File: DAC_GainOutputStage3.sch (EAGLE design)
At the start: 55 parts, among them J1 1935190, J3 SJ-63033A

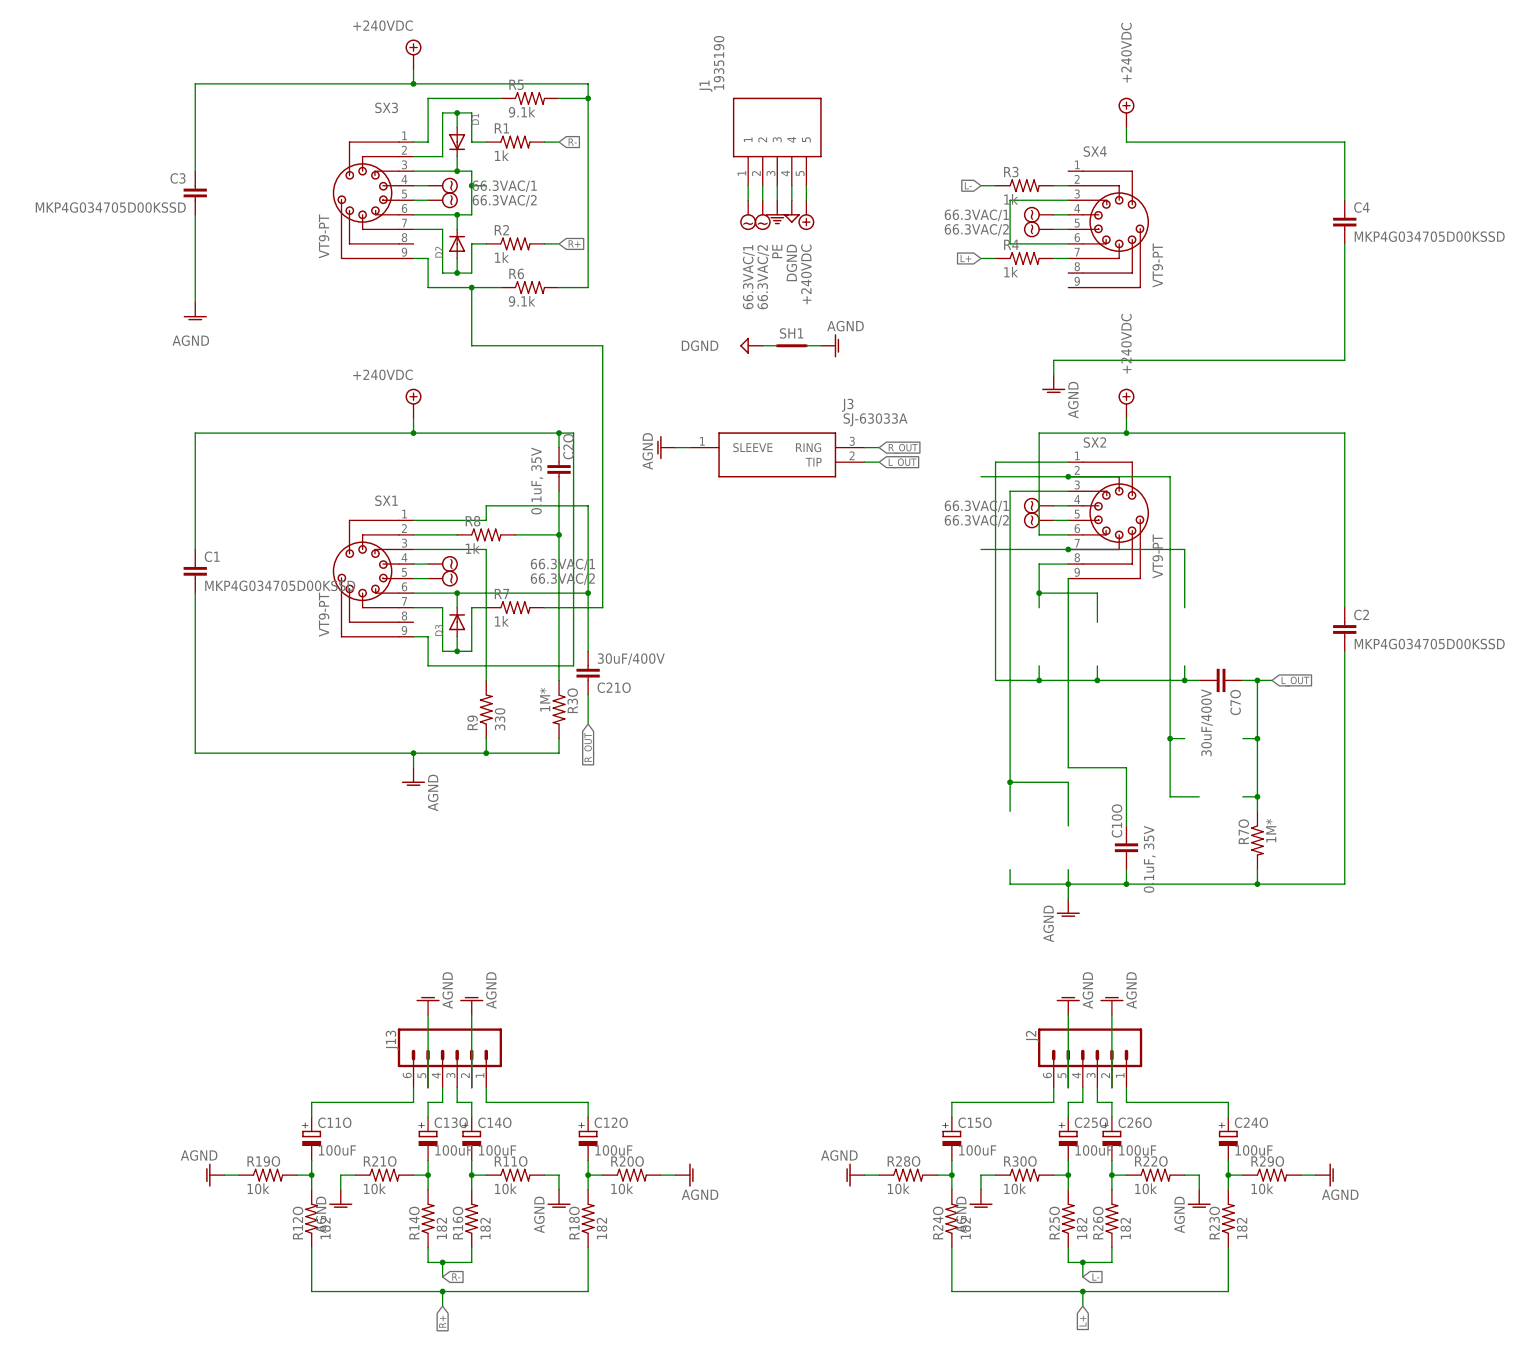
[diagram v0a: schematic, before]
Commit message: Finished schematic and working layout
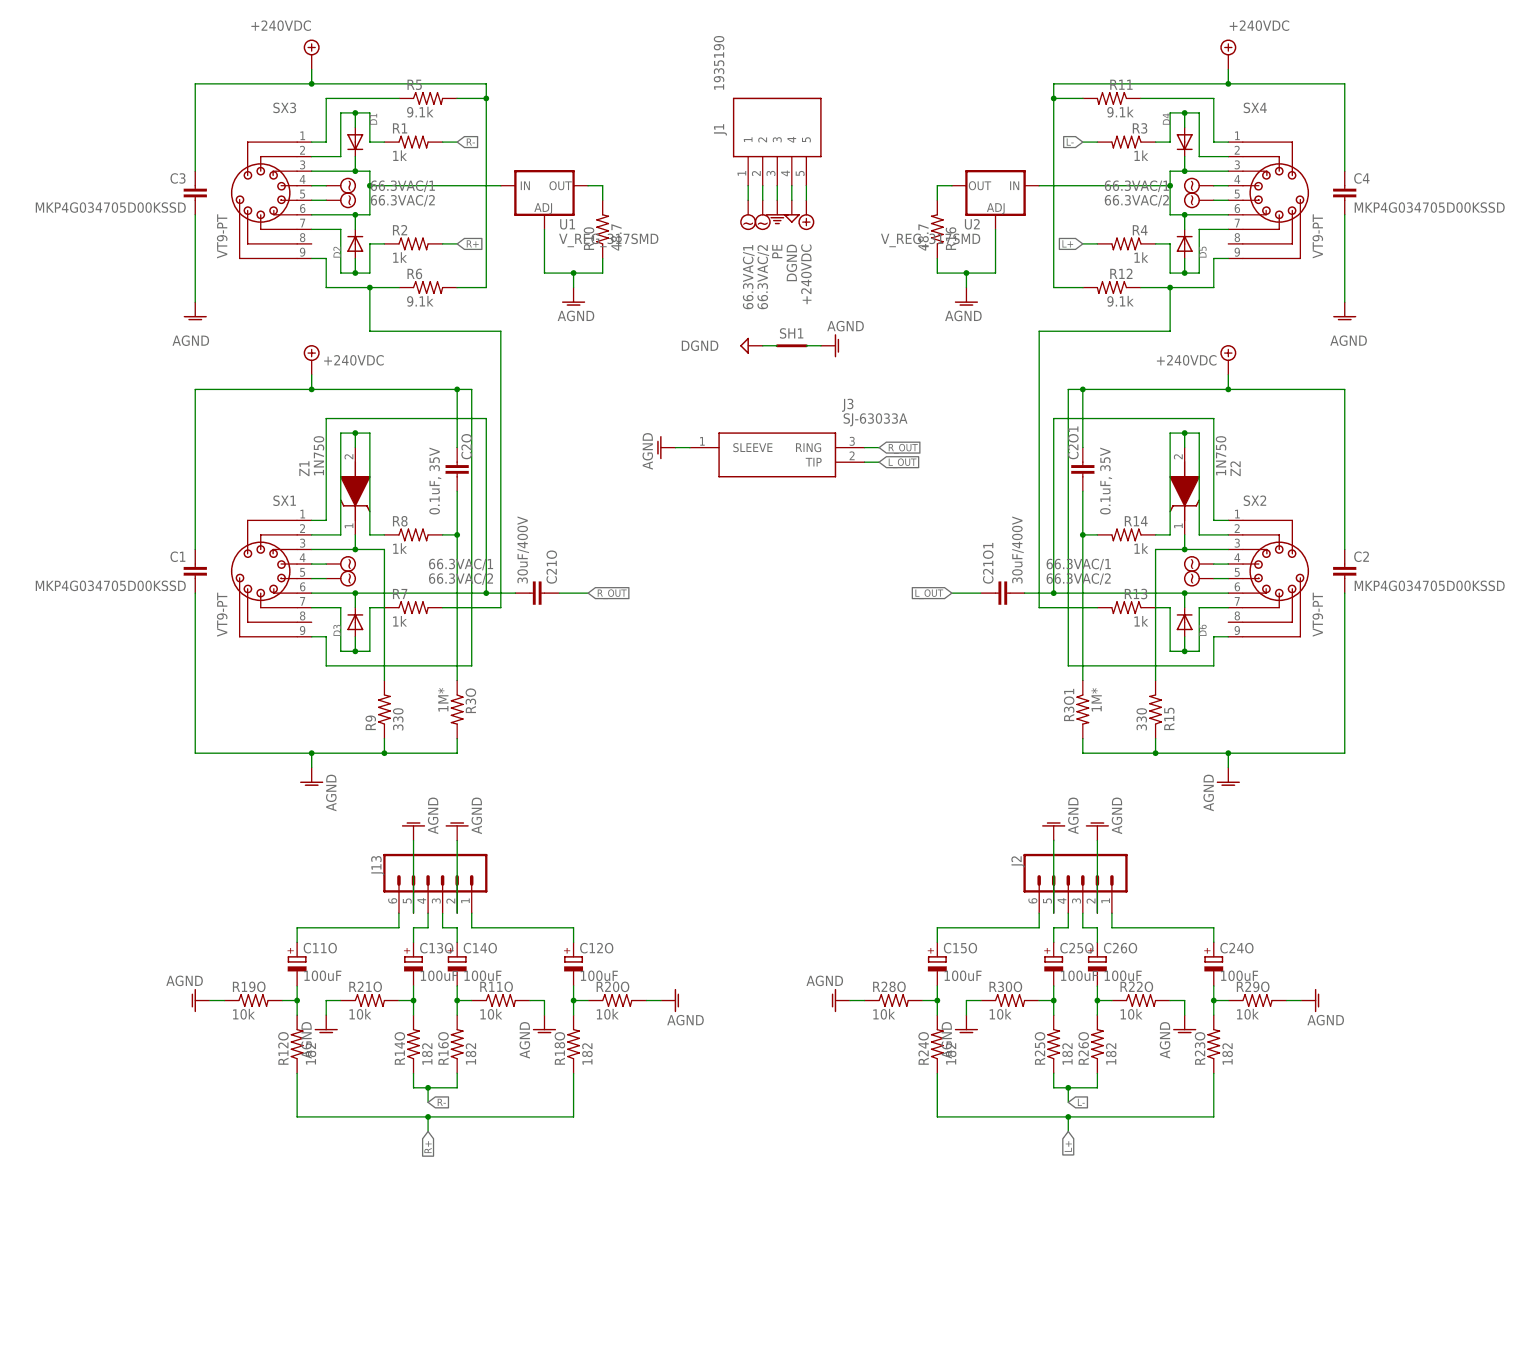
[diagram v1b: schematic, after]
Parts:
- removed C10O: 0.1uF, 35V, Dual Mono Amp Library:MKS4B031002A00JC00
- removed C7O: 30uF/400V, Dual Mono Amp Library:DCP4G053006ID2KSSD
- removed R7O: 1M*, Dual Mono Amp Library:LR1F1M0
- added C21O1: 30uF/400V, Dual Mono Amp Library:DCP4G053006ID2KSSD
- added C2O1: 0.1uF, 35V, Dual Mono Amp Library:MKS4B031002A00JC00
- added D4, D5, D6: (no value), adafruit:DIODEDO-1N4148
- added R10, R16: 48.7, rcl:R-US_0207/10
- added R11, R12: 9.1k, rcl:R-US_0207/10
- added R13, R14: 1k, rcl:R-US_0207/10
- added R15: 330, rcl:R-US_0207/10
- added R3O1: 1M*, Dual Mono Amp Library:LR1F1M0
- added U1, U2: V_REG_317SMD, SparkFun-IC-Power:V_REG_317SMD
- added Z1, Z2: 1N750, 1N750:1N750
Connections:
- new net N$29: D6.A, R13.1, SX2.7
- new net N$37: R10.2, U1.OUT
- new net N$38: R16.2, U2.OUT
- net +240VDC: now also C2O1.1, R11.2, R12.2, SX2.9; no longer SX2.6
- net AGND: now also R10.1, R15.1, R16.1, R3O1.2, U1.ADJ, U2.ADJ; no longer C10O.2, R7O.2
- net L+: now also R4.2; no longer R4.1
- net L-: now also R3.2; no longer R3.1
- net L_OUT: now also C21O1.1; no longer C7O.1, R7O.1
- net N$14: now also R14.1, SX2.2, Z2.A; no longer R3.2, SX4.2
- net N$17: now also C2O1.2, R14.2, R3O1.1; no longer R4.2, SX4.7
- net N$2: now also Z1.A
- net N$22: now also U1.IN
- net N$26: now also Z1.K
- net N$27: now also R15.2, SX2.3, Z2.K; no longer SX4.3, SX4.6
- net N$3: now also C21O1.2, D6.C, SX2.1, SX2.6; no longer SX2.7
- net N$4: now also D4.A, R3.1, SX4.2; no longer SX2.8
- net N$5: now also D5.A, R4.1, SX4.7; no longer C7O.2, SX2.1
- net N$7: now also D4.C, D5.C, SX4.3, SX4.6, U2.IN; no longer SX2.2
- net N$8: now also R11.1, SX4.1; no longer SX2.3
- net N$9: now also R12.1, R13.2, SX4.9; no longer C10O.1, SX2.9
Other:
- moved on the sheet: C11O, C12O, C13O, C14O, C15O, C2, C21O, C24O, C25O, C26O, C2O, C4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
